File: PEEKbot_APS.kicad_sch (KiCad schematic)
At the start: 34 parts, among them J1 Conn_01x02, J2 Conn_01x05, J3 0705430109, J4 0705430109, SW1 SW_DIP_x04, U1 SN65HVD72DRBR, U2 DRV5011, U3 STM32G071CBT6, U4 DRV5011

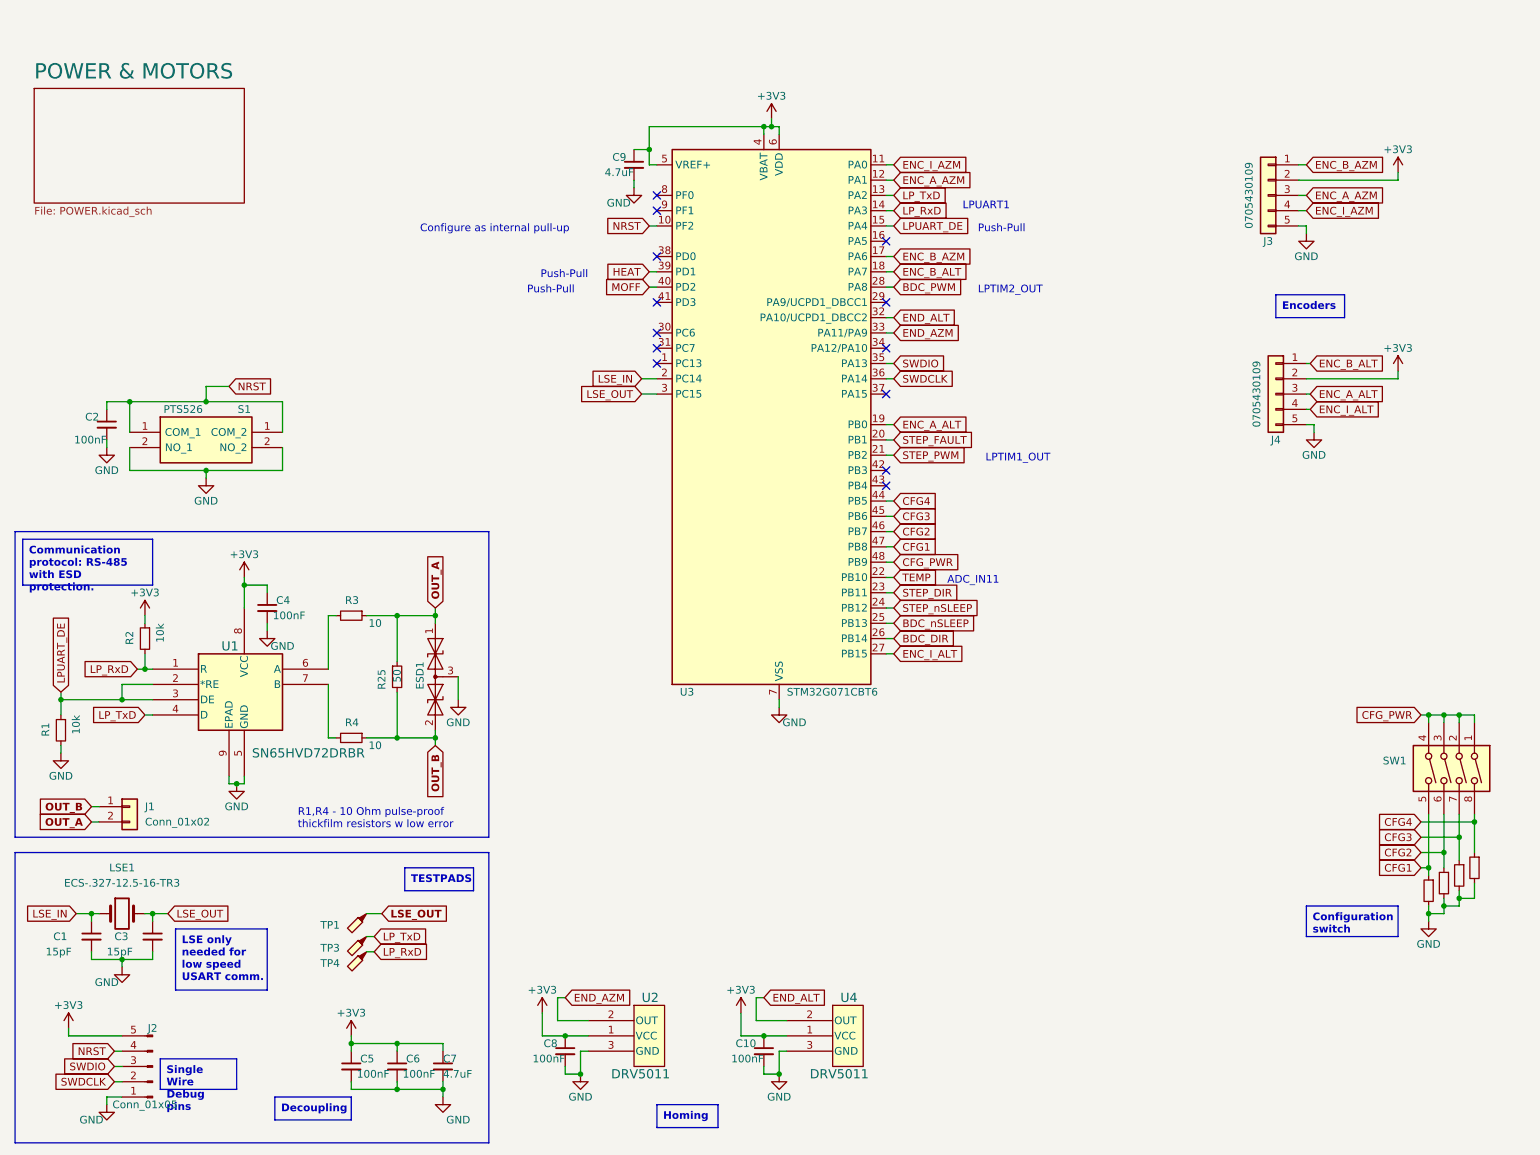
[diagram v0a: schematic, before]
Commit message: Add files via upload
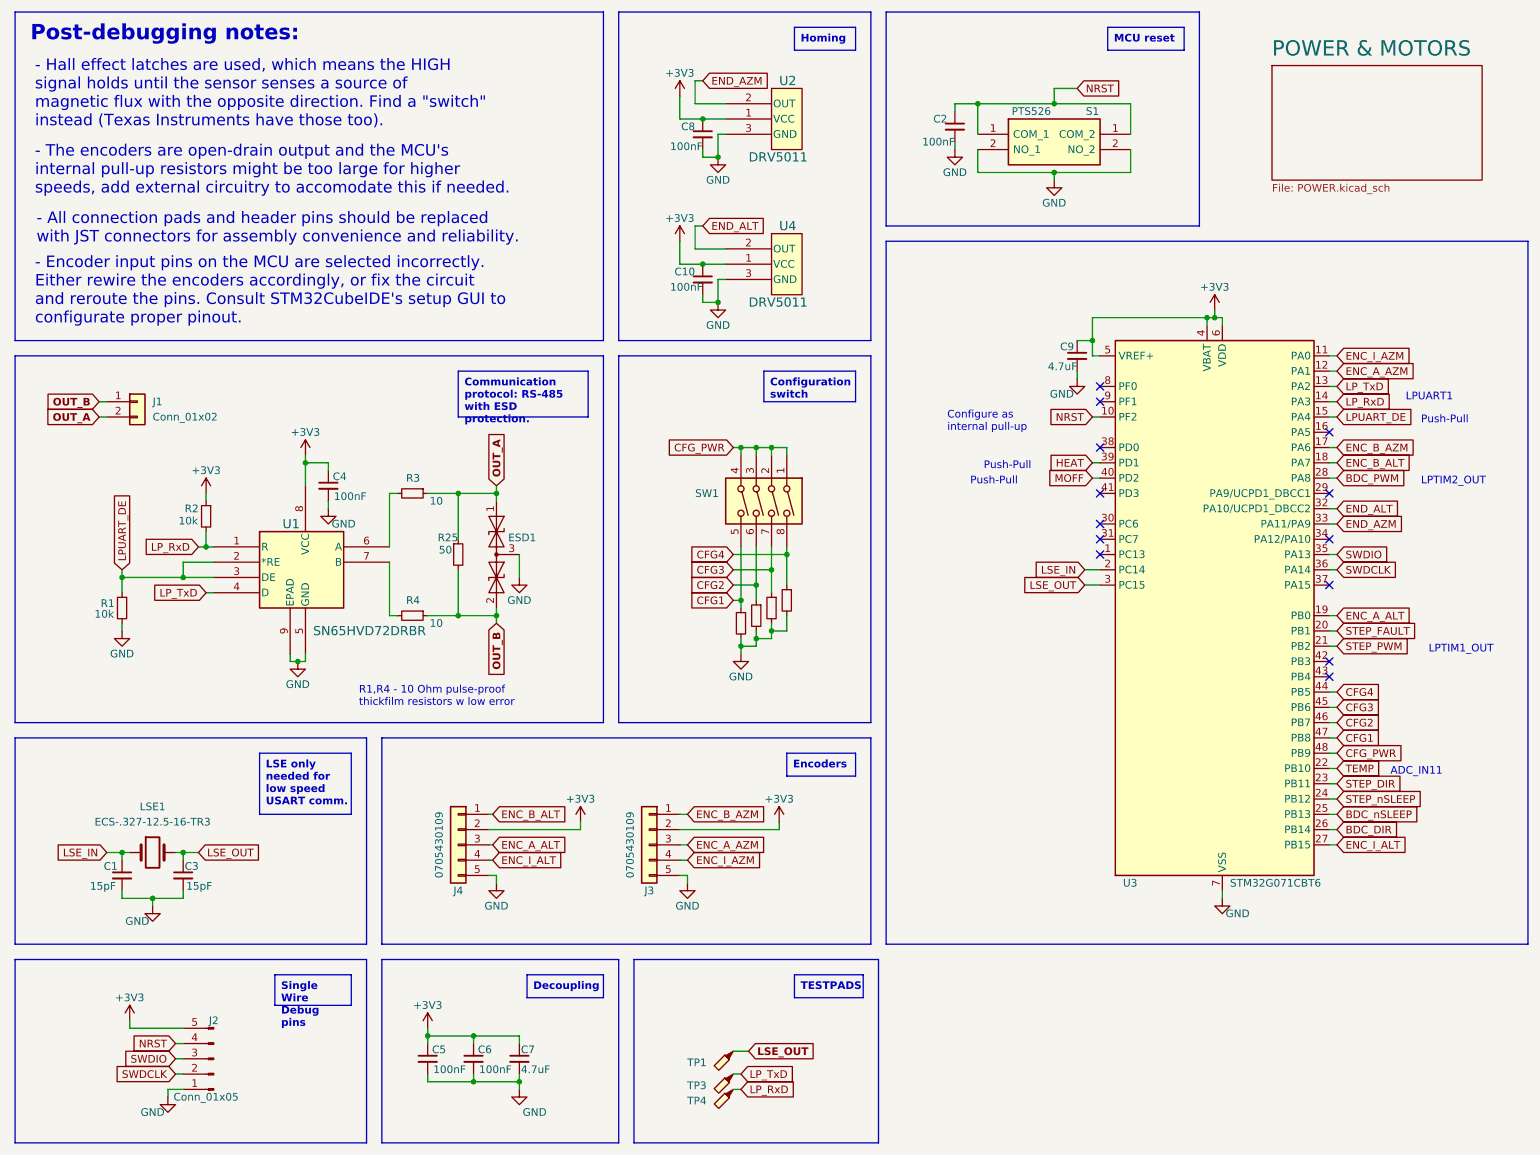
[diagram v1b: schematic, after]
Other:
- note added: "- All connection pads and header pins should be replaced with JST connectors for assembly convenience and reliability."
- note added: "- Encoder input pins on the MCU are selected incorrectly. Either rewire the encoders accordingly, or fix the circuit and reroute the pins. Consult STM32CubeIDE's setup GUI to configurate proper pinout."
- note added: "- Hall effect latches are used, which means the HIGH signal holds until the sensor senses a source of magnetic flux with the opposite direction. Find a "switch" instead (Texas Instruments have those too)."
- note added: "- The encoders are open-drain output and the MCU's internal pull-up resistors might be too large for higher speeds, add external circuitry to accomodate this if needed."
- note added: "Post-debugging notes:"
- moved on the sheet: C1, C10, C2, C3, C4, C5, C6, C7, C8, C9, ESD1, J1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
